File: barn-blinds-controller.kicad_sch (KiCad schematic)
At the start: 20 parts, among them J1 Power Input, J2 Motor 1 Output, J3 Motor 2 Output, J4 Motor 3 Output, M1 Blind 1, M2 Blind 2, M3 Blind 3, U1 ESP32-DevKitC, U2 TB6612, U3 TB6612, U4 LM2596 Buck Converter 12-5

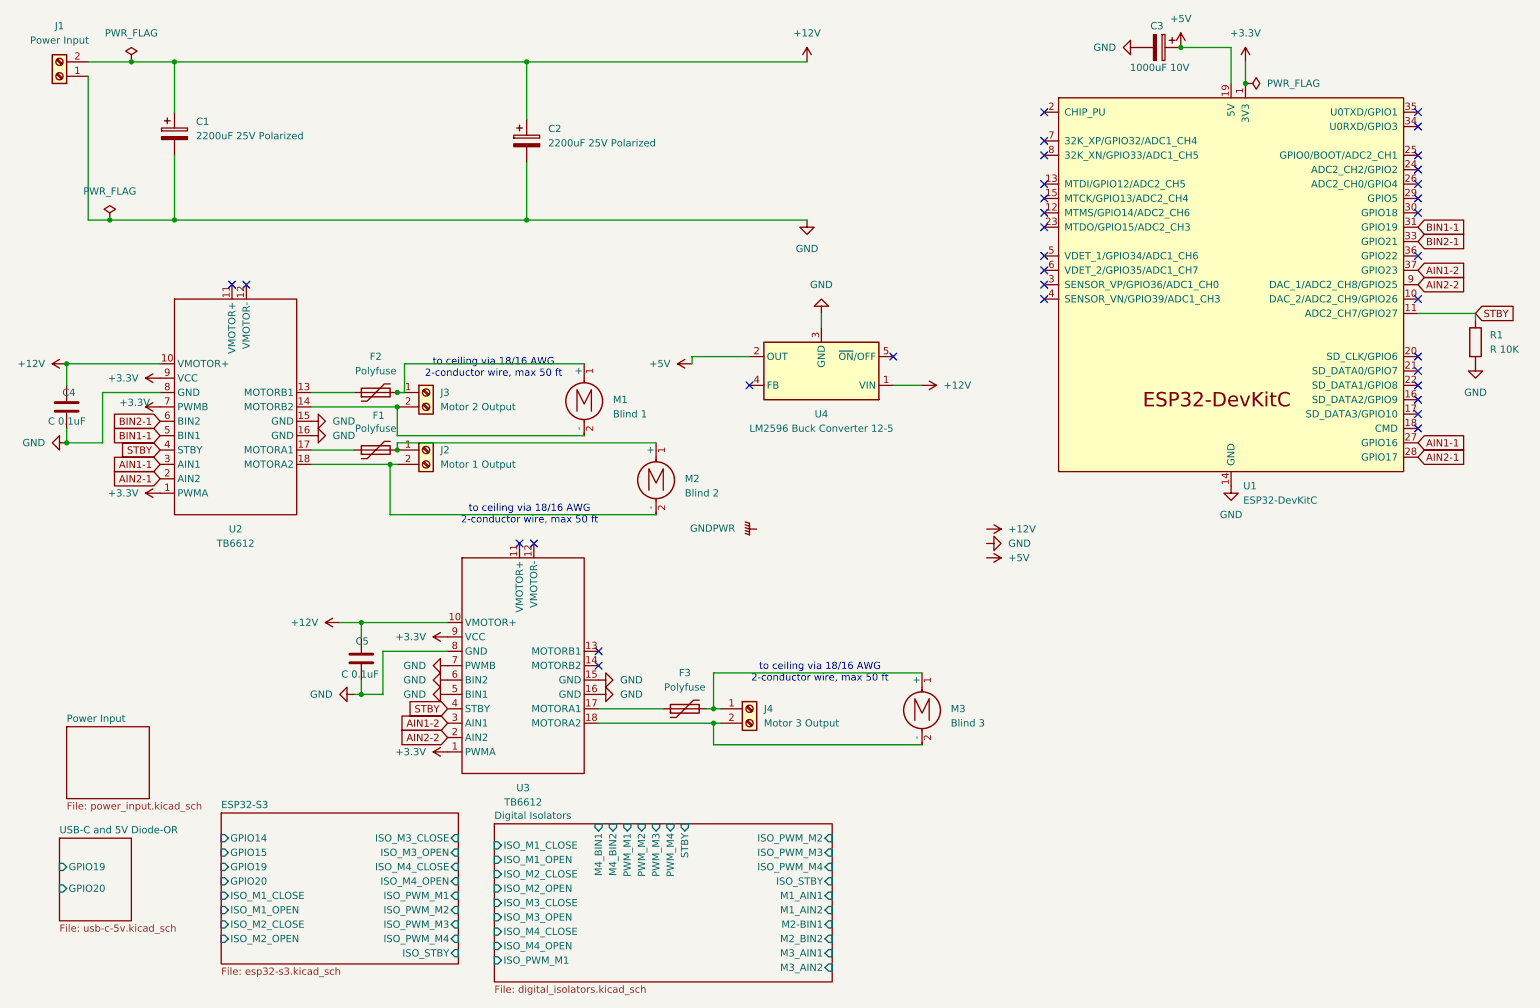
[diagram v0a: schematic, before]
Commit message: Started running traces
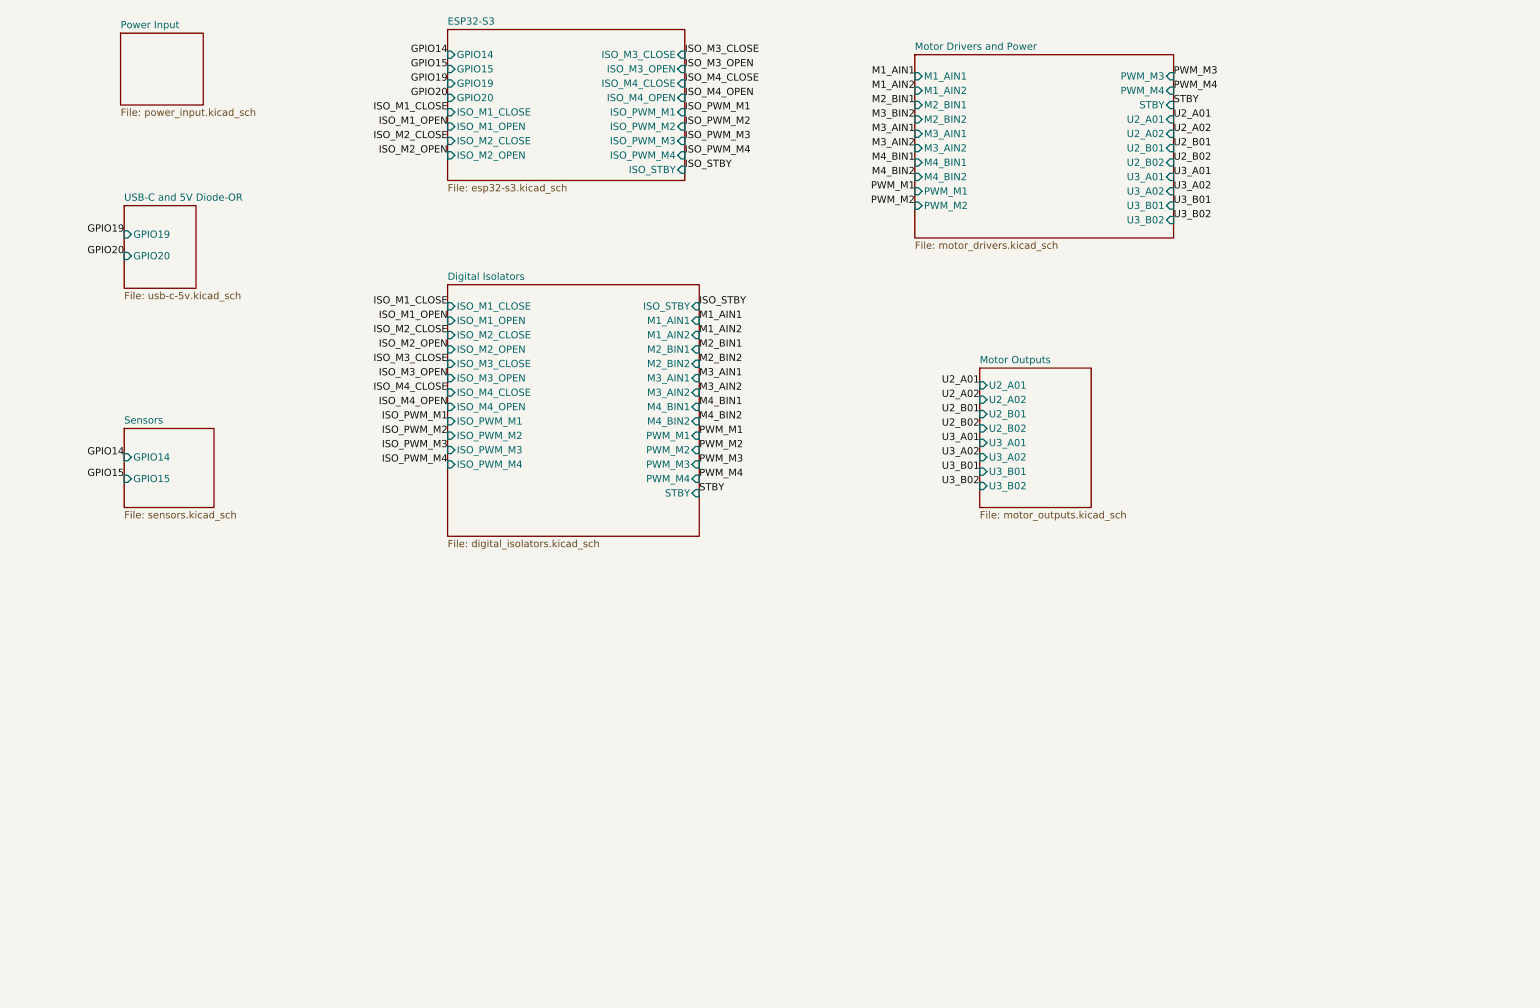
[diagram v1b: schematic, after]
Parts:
- removed C1, C2: 2200uF 25V Polarized, symbol Device:C_Polarized
- removed C3: 1000uF 10V, symbol Device:C_Polarized
- removed C4, C5: C 0.1uF, symbol Device:C
- removed F1, F2, F3: Polyfuse, symbol Device:Polyfuse
- removed J1: Power Input, symbol Connector:Screw_Terminal_01x02
- removed J2: Motor 1 Output, symbol Connector:Screw_Terminal_01x02
- removed J3: Motor 2 Output, symbol Connector:Screw_Terminal_01x02
- removed J4: Motor 3 Output, symbol Connector:Screw_Terminal_01x02
- removed M1: Blind 1, symbol Motor:Motor_DC
- removed M2: Blind 2, symbol Motor:Motor_DC
- removed M3: Blind 3, symbol Motor:Motor_DC
- removed R1: R 10K, symbol Device:R
- removed U1: ESP32-DevKitC, PCM_Espressif:ESP32-DevKitC, symbol PCM_Espressif:ESP32-DevKitC
- removed U2, U3: TB6612, symbol New_Library:TB6612_Breakout
- removed U4: LM2596 Buck Converter 12-5, Package_TO_SOT_SMD:TO-263-5_TabPin3, symbol Regulator_Switching:LM2596S-3.3
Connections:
- no-connect marks 34 -> 0
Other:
- added sheet Motor Drivers and Power (motor_drivers.kicad_sch)
- added sheet Motor Outputs (motor_outputs.kicad_sch)
- added sheet Sensors (sensors.kicad_sch)
- sheet Digital Isolators ports: added M2_BIN1; removed M2-BIN1
- note removed: "to ceiling via 18/16 AWG 2-conductor wire, max 50 ft"
